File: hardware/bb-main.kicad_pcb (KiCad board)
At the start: 2 copper layers, 50.5 x 19 mm, 28 parts, among them P1 USB_B, P2 PICkit3, P3 OLED, SW1 SW_PUSH, U1 BU33TD3WG-TR, U2 PIC16(L)F1455-I/SL

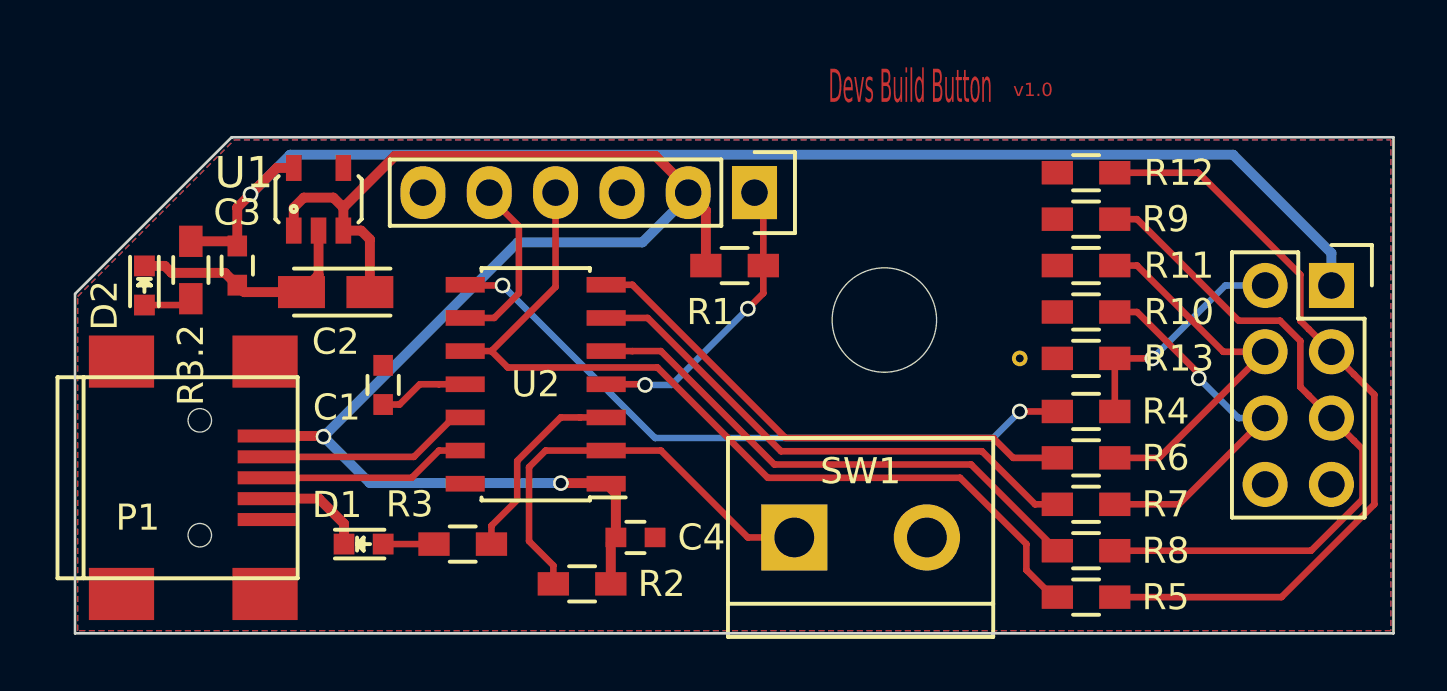
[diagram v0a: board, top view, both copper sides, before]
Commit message: Board final rev 1.0
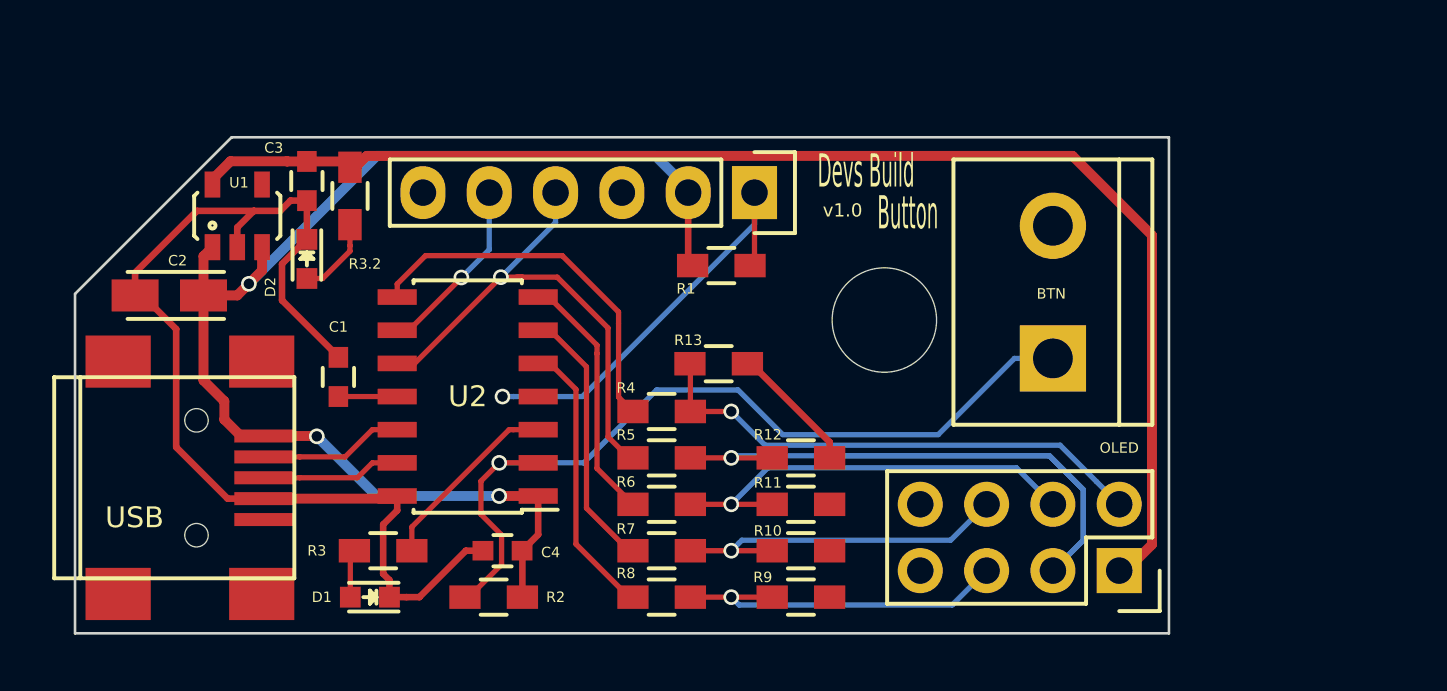
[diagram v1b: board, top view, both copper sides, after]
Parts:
- removed ?: , Housings_Proj:VIA-0.6mm
- moved R9 18.1 mm to (82.8, 86.6), turned to 180 degrees
- moved R5 17.1 mm to (77.5, 81.3)
- moved R6 16.4 mm to (77.5, 83.1)
- moved R8 16.4 mm to (77.5, 86.6)
- moved R7 16.4 mm to (77.5, 84.8)
- moved R4 16.3 mm to (77.5, 79.5)
- moved R12 15.4 mm to (82.8, 81.3), turned to 180 degrees
- moved R10 14.2 mm to (82.8, 84.8), turned to 180 degrees
- moved R11 14.2 mm to (82.8, 83.1), turned to 180 degrees
- moved R13 14.1 mm to (79.7, 77.7), turned to 180 degrees
- moved OLED 13.6 mm to (95.0, 85.6), turned to 180 degrees
- moved BTN 11.9 mm to (92.5, 74.9), turned to 90 degrees
- moved R3.2 6.72 mm to (65.5, 71.2)
- moved C2 6.37 mm to (58.6, 75.1)
- moved D2 6.31 mm to (63.9, 73.7)
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- renumbered SW1 to BTN, P3 to OLED, P1 to USB
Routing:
- net GND: track 13.2 -> 47.9 mm
- net /BUT_1: track 16.7 -> 32.7 mm, vias 0 -> 1
- net /ICSPDAT/OLED_SCK: track 34.3 -> 20.0 mm, vias 0 -> 1
- net /~RES~: track 26.4 -> 13.6 mm, vias 0 -> 1
- net /OLED_SDO: track 25.5 -> 14.4 mm, vias 2 -> 0
- net /SDO: track 8.95 -> 19.7 mm
- net /OLED_D/~C~: track 20.0 -> 9.83 mm
- net /OLED_~CS~: track 20.2 -> 10.3 mm
- net +5V: track 60.8 -> 50.9 mm, vias 2 -> 3
- net /OLED_~RES~: track 20.4 -> 10.8 mm
- net /~MCLR~: track 11.6 -> 16.6 mm, vias 2 -> 1
- net /SCK: track 30.1 -> 35.1 mm, vias 0 -> 1
- net Net-(P1-Pad3): track 8.00 -> 5.33 mm
- net Net-(P1-Pad2): track 8.19 -> 5.52 mm
- net /D/~C~: track 14.6 -> 16.6 mm, vias 0 -> 1
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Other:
- board size 50.5 x 19 mm -> 41.9 x 19 mm
- net class Default: trace_width 0.254 -> 0.2032
- net class Power: trace_width 0.381 -> 0.254
- rule via_min_size: 0.4 -> 0.3302
- board text added: "Button"
- board text added: "Devs Build"
- board text removed: "Devs Build Button"
